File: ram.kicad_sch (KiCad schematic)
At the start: 8 parts, among them U501 MT48LC16M16A2

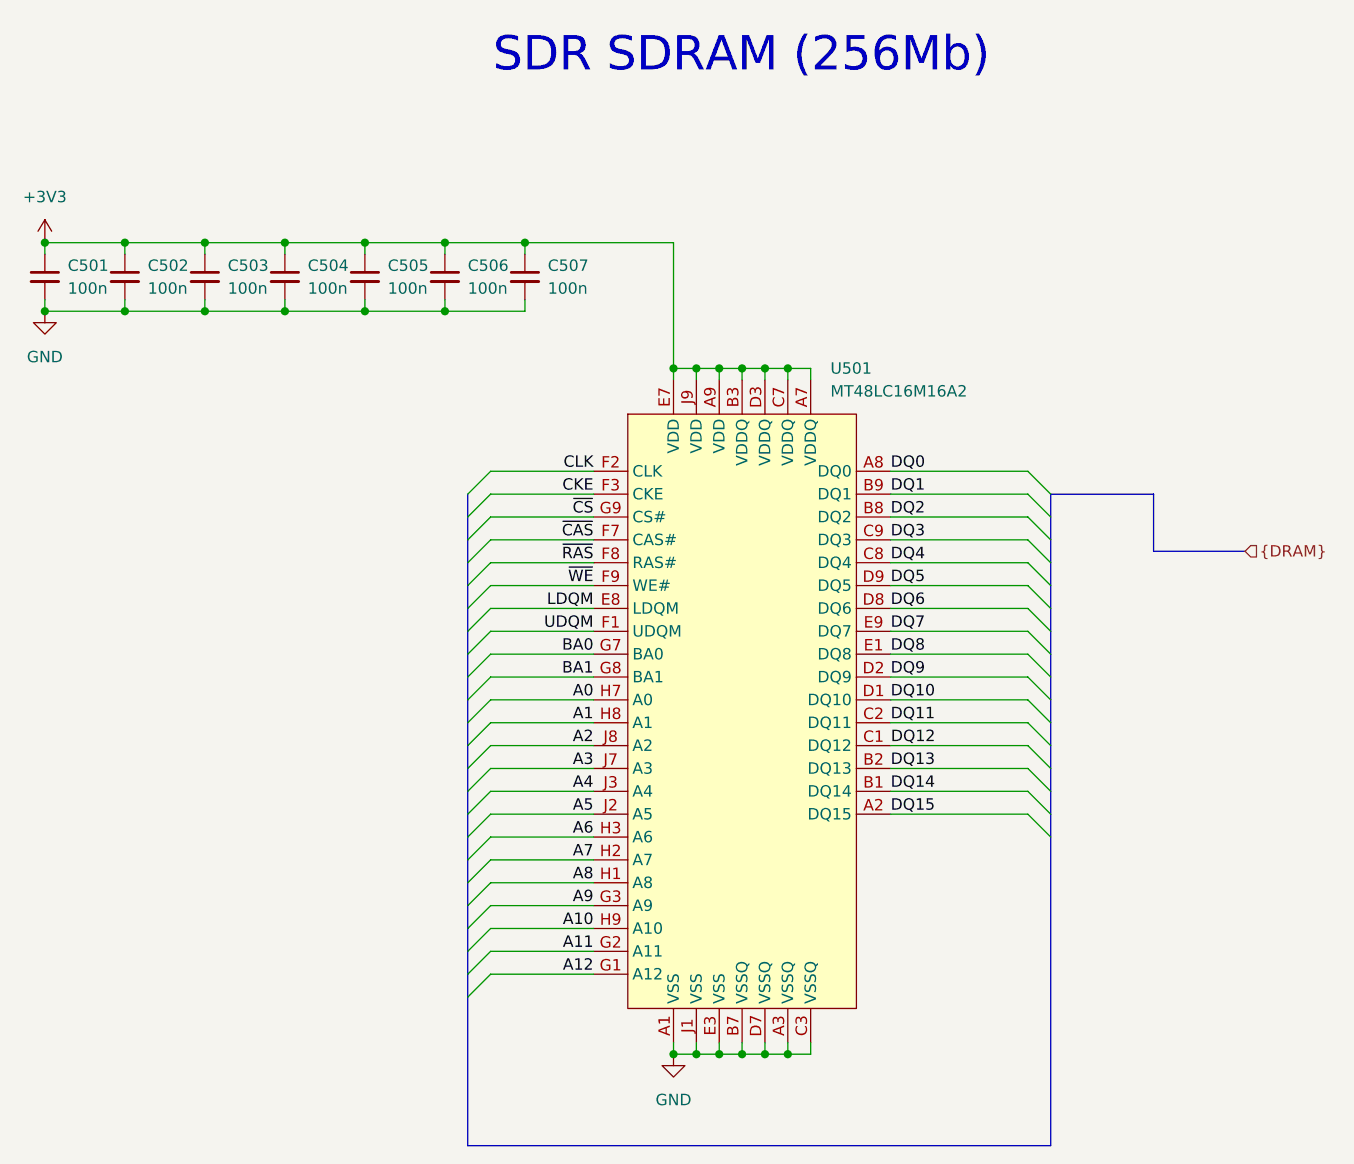
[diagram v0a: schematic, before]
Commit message: First whole routing
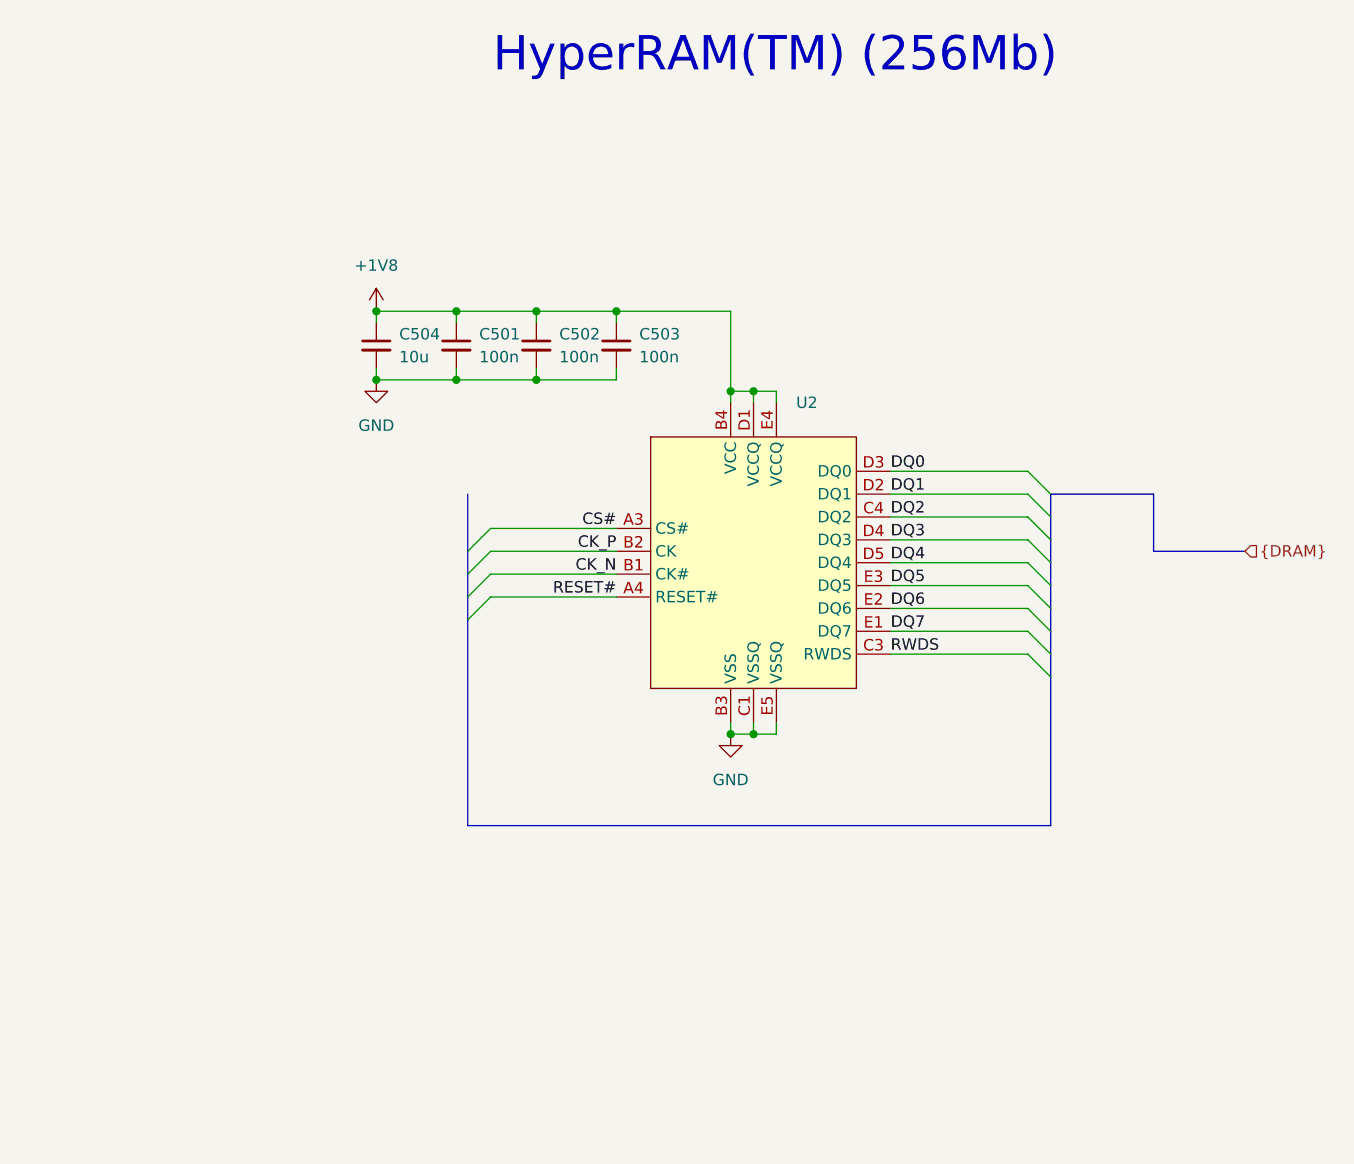
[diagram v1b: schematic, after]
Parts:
- removed C505, C506, C507: 100n, Capacitor_SMD:C_0201_0603Metric, symbol Device:C_Small
- removed U501: MT48LC16M16A2, Package_BGA_Extra:Micron_VFBGA-64_8.0x8.0mm_Layout9x9_P0.8mm, symbol Memory_RAM_Extra:MT48LC16M16A2
- added U2: ~, Package_BGA_Extra:FBGA-25_8x6mm_Layout5x5_P1mm, symbol Memory_RAM_Extra:S80KS2562
- C501, C502, C503: footprint Capacitor_SMD:C_0201_0603Metric -> Capacitor_SMD:C_0402_1005Metric
- C504: value 100n -> 10u; footprint Capacitor_SMD:C_0201_0603Metric -> Capacitor_SMD:C_0402_1005Metric
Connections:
- net DQ0: now also U2.D3 (DQ0)
- net DQ1: now also U2.D2 (DQ1)
- net DQ2: now also U2.C4 (DQ2)
- net DQ3: now also U2.D4 (DQ3)
- net DQ4: now also U2.D5 (DQ4)
- net DQ5: now also U2.E3 (DQ5)
- net DQ6: now also U2.E2 (DQ6)
- net DQ7: now also U2.E1 (DQ7)
- net GND: now also U2.B3 (VSS), U2.C1 (VSSQ), U2.E5 (VSSQ)
- net +3V3 renamed +1V8
- net +1V8: now also U2.B4 (VCC), U2.D1 (VCCQ), U2.E4 (VCCQ)
- new net: U2.A2 (RFU), U2.A5 (RFU), U2.B5 (RFU), U2.C2 (RFU), U2.C5 (RFU)
- new net CK_N: U2.B1 (CK#)
- new net CK_P: U2.B2 (CK)
- new net CS#: U2.A3 (CS#)
- new net RESET#: U2.A4 (RESET#)
- new net RWDS: U2.C3 (RWDS)
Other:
- note added: "HyperRAM(TM) (256Mb)"
- note removed: "SDR SDRAM (256Mb)"
- moved on the sheet: C501, C502, C503
